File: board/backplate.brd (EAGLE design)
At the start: 68.2 x 43.2 mm, 22 parts, among them IC1 MAX7219CNG, IC2 MAX7219CNG, IC3 MAX7219CNG, IC4 MAX7219CNG

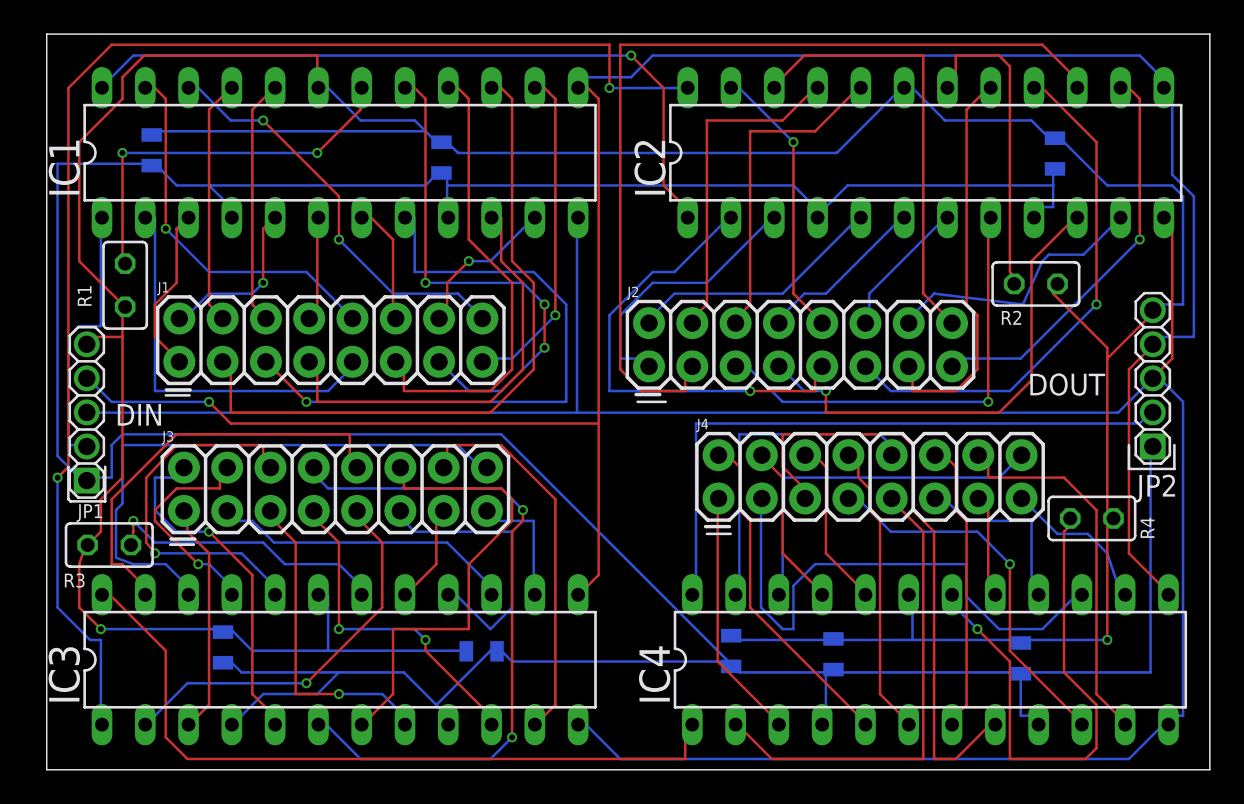
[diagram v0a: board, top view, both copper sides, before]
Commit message: backplight v2
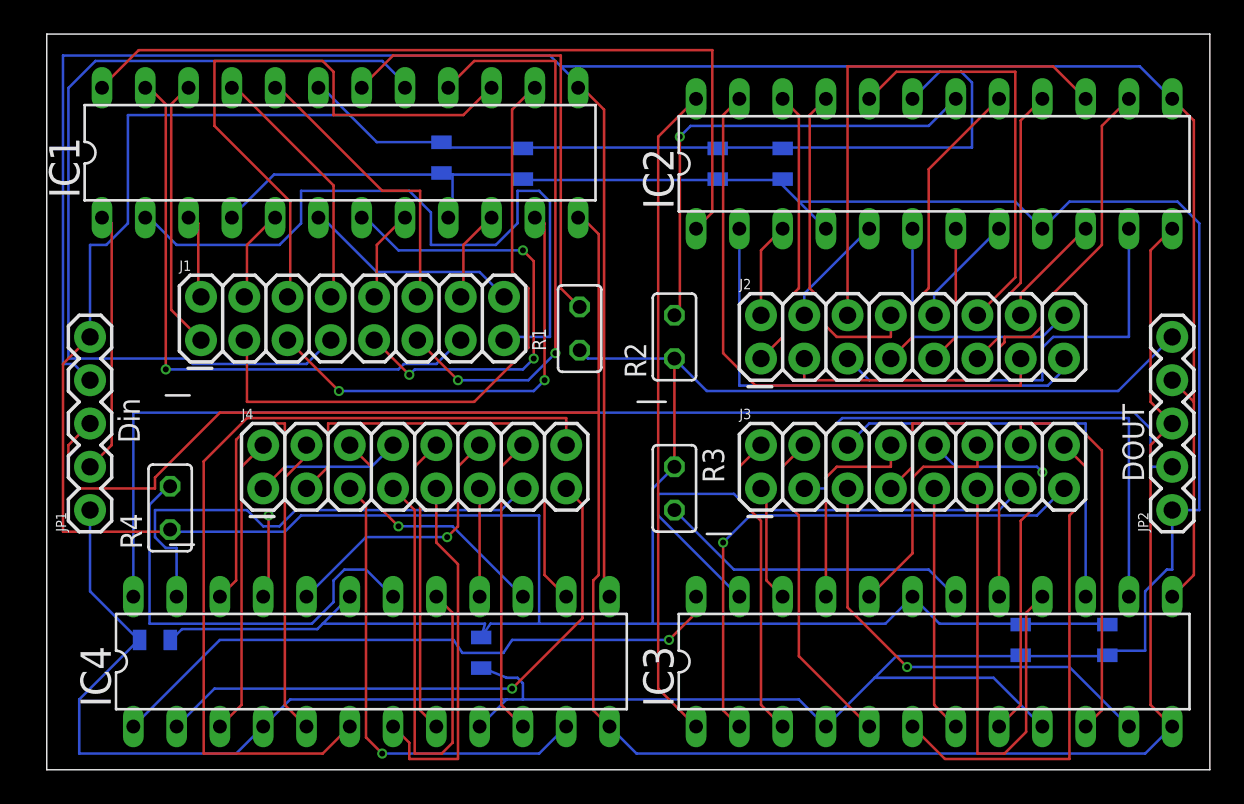
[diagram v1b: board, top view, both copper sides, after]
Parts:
- JP1, JP2: device pinhead:1_05X2MM -> SparkFun-Connectors:1X05
- moved C4 58.5 mm to (57.1, 7.62)
- moved R4 54.1 mm to (7.24, 15.4), turned to 90 degrees
- moved C8 40.6 mm to (39.4, 35.6)
- moved IC3 34.9 mm to (52.1, 6.35)
- moved C7 34.1 mm to (27.9, 35.6)
- moved J3 33.9 mm to (41.9, 16.5)
- moved C6 33.8 mm to (6.35, 7.62), turned to 0 degrees
- moved R3 33.3 mm to (36.8, 16.5), turned to 270 degrees
- moved IC4 32.8 mm to (19.1, 6.35)
- moved C3 32.2 mm to (43.2, 35.6)
- moved C5 28.7 mm to (62.2, 7.62)
- moved R1 26.8 mm to (31.3, 25.9)
- moved J4 26.7 mm to (12.7, 16.5)
- moved R2 21.4 mm to (36.8, 25.4), turned to 90 degrees
- moved JP2 7.81 mm to (66.0, 15.2)
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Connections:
- removed net N$13 (its old number): IC1.7, J1.12
- removed net N$17: IC1.14, J1.15
- removed net N$19 (its old number): IC2.3, J2.1
- removed net N$20 (its old number): IC2.5, J2.2
- removed net N$29: IC2.7, J2.12
- removed net N$31: IC2.11, J2.14
- removed net N$33 (its old number): IC2.14, J2.15
- removed net N$34: IC2.6, J2.8
- removed net N$40 (its old number): IC3.8, J3.5
- removed net N$41 (its old number): IC3.20, J3.6
- removed net N$58 (its old number): IC4.20, J4.6
- removed net N$59 (its old number): IC4.10, J4.7
- removed net N$63: IC4.7, J4.12
- removed net N$65: IC4.11, J4.14
- removed net N$68: IC4.6, J4.8
- new net N$2: IC1.23, J1.13
- new net N$28: IC2.5, J2.4
- new net N$35: IC2.23, J2.13
- new net N$45: IC3.6, J3.16
- new net N$62: IC4.11, J4.5
- new net N$69: IC4.10, J4.14
- new net N$71: IC1.20, J1.12
- new net N$72: IC4.5, J4.4
- new net N$73: IC4.8, J4.10
- new net N$74: IC4.14, J4.3
- new net N$76: IC4.23, J4.13
- new net N$77: IC4.21, J4.8
- new net N$78: IC4.15, J4.6
- new net N$79: IC4.17, J4.7
- new net N$80: IC4.22, J4.1
- net N$10: now also IC1.8; no longer IC1.23
- net N$11: now also IC1.14, J1.3; no longer IC1.2, J1.9
- net N$14: now also IC1.21, J1.8; no longer IC1.17, J1.13
- net N$15: now also IC1.15, J1.6; no longer IC1.11, J1.14
- net N$16: now also IC1.17, J1.7; no longer IC1.22, J1.16
- net N$18: now also IC1.22, J1.1; no longer IC1.6, J1.8
- net N$21: now also IC2.20, J2.12; no longer IC2.15, J2.3
- net N$22: now also IC2.2, J2.15; no longer IC2.21, J2.4
- net N$23: now also IC2.11; no longer IC2.8
- net N$24: now also IC2.6, J2.16; no longer IC2.20, J2.6
- net N$25: now also IC2.7, J2.9; no longer IC2.10, J2.7
- net N$26: now also IC2.3, J2.2; no longer IC2.23, J2.10
- net N$27: now also IC2.10, J2.14; no longer IC2.2, J2.9
- net N$3: now also IC1.2, J1.15; no longer IC1.3, J1.1
- net N$30: now also IC2.8, J2.10; no longer IC2.17, J2.13
- net N$32: now also IC2.14, J2.3; no longer IC2.22, J2.16
- net N$36: now also IC2.21, J2.8; no longer IC3.3, J3.1
- net N$37: now also IC2.15, J2.6; no longer IC3.5, J3.2
- net N$38: now also IC2.17, J2.7; no longer IC3.15, J3.3
- net N$39: now also IC2.22, J2.1; no longer IC3.21, J3.4
- net N$4: now also IC1.11, J1.5; no longer IC1.5, J1.2
- net N$42: now also IC3.20, J3.12; no longer IC3.10, J3.7
- net N$43: now also IC3.2, J3.15; no longer IC3.23, J3.10
- net N$44: now also IC3.11, J3.5; no longer IC3.2, J3.9
- net N$46: now also J3.9; no longer J3.12
- net N$47: now also IC3.3, J3.2; no longer IC3.17, J3.13
- net N$48: now also IC3.10; no longer IC3.11
- net N$49: now also IC3.5, J3.4; no longer IC3.22, J3.16
- net N$5: now also IC1.6, J1.16; no longer IC1.15, J1.3
- net N$50: now also IC3.8, J3.10; no longer IC3.14, J3.15
- net N$51: now also IC3.14, J3.3; no longer IC3.6, J3.8
- net N$53: now also IC3.23, J3.13; no longer IC4.3, J4.1
- net N$54: now also IC3.21, J3.8; no longer IC4.5, J4.2
- net N$55: now also IC3.15, J3.6; no longer IC4.15, J4.3
- net N$56: now also IC3.17, J3.7; no longer IC4.21, J4.4
- net N$57: now also IC3.22, J3.1; no longer IC4.8, J4.5
- net N$6: now also IC1.7, J1.9; no longer IC1.21, J1.4
- net N$60: now also IC4.20, J4.12; no longer IC4.23, J4.10
- net N$61: now also J4.15; no longer J4.9
- net N$64: now also IC4.6, J4.16; no longer IC4.17, J4.13
- net N$66: now also IC4.7, J4.9; no longer IC4.22, J4.16
- net N$67: now also IC4.3, J4.2; no longer IC4.14, J4.15
- net N$7: now also IC1.3, J1.2; no longer IC1.8, J1.5
- net N$8: now also IC1.10, J1.14; no longer IC1.20, J1.6
- net N$9: now also IC1.5, J1.4; no longer IC1.10, J1.7
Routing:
- net N$64: track 6.34 -> 50.3 mm
- net N$20: track 79.0 -> 38.7 mm, vias 2 -> 0
- net DOUT: track 37.2 -> 74.4 mm
- net N$2: track 0.00 -> 35.2 mm, vias 0 -> 1
- net N$35: track 0.00 -> 35.2 mm
- net N$3: track 9.89 -> 42.7 mm
- net N$7: track 37.7 -> 5.08 mm, vias 1 -> 0
- net N$45: track 0.00 -> 29.3 mm
- net N$76: track 0.00 -> 28.9 mm
- net N$16: track 24.3 -> 53.2 mm, vias 2 -> 0
- net N$21: track 53.2 -> 24.4 mm
- net N$57: track 35.5 -> 6.88 mm
- net N$62: track 0.00 -> 27.8 mm, vias 0 -> 1
- net N$79: track 0.00 -> 27.5 mm
- net N$74: track 0.00 -> 27.4 mm
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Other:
- board text added: "Din"
- board text removed: "DIN"
